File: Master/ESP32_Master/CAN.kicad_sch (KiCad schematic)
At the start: 6 parts, among them U11 ISO1050DUBR

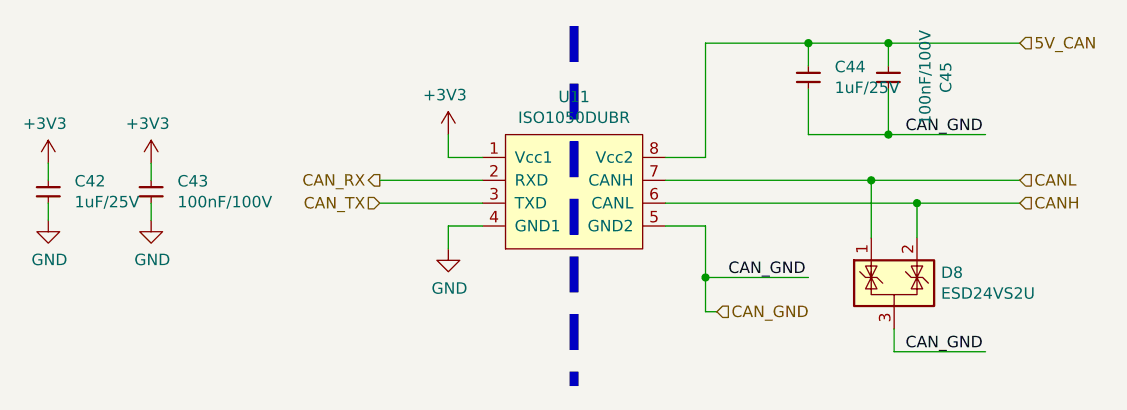
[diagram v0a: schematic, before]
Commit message: Add files via upload
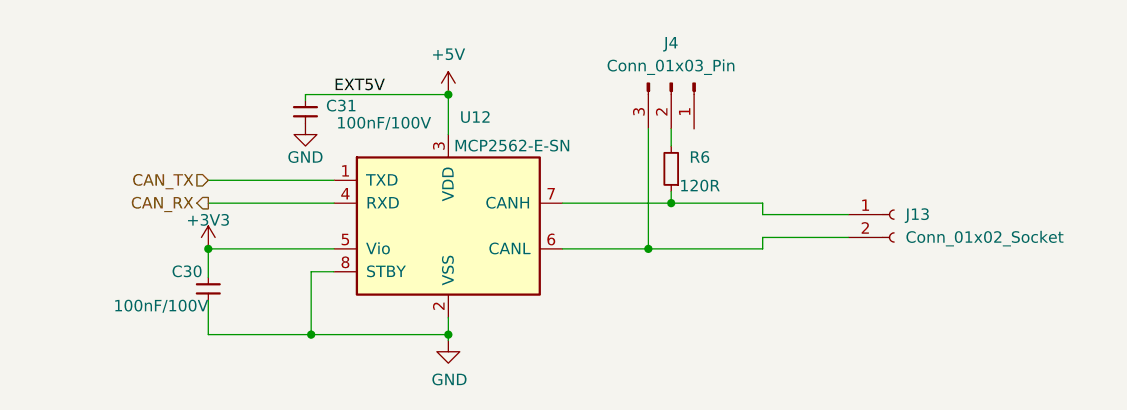
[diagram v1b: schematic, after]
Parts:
- removed C42, C44: 1uF/25V, Capacitor_SMD:C_0603_1608Metric, symbol Device:C
- removed C43, C45: 100nF/100V, Capacitor_SMD:C_0603_1608Metric, symbol Device:C
- removed D8: ESD24VS2U, Package_TO_SOT_SMD:SOT-23, symbol Power_Protection:SZNUP2105L
- removed U11: ISO1050DUBR, Package_SO:SOP-8_6.62x9.15mm_P2.54mm, symbol ENNOID:ISO1050DUBR
- added C30, C31: 100nF/100V, Capacitor_SMD:C_0603_1608Metric, symbol Device:C
- added J13: Conn_01x02_Socket, Connector_PinSocket_2.54mm:PinSocket_1x02_P2.54mm_Vertical, symbol Connector:Conn_01x02_Socket
- added J4: Conn_01x03_Pin, Connector_PinHeader_2.54mm:PinHeader_1x03_P2.54mm_Vertical, symbol Connector:Conn_01x03_Pin
- added R6: 120R, Resistor_SMD:R_0603_1608Metric, symbol Device:R_Small
- added U12: MCP2562-E-SN, Package_SO:SOIC-8_3.9x4.9mm_P1.27mm, symbol Interface_CAN_LIN:MCP2562-E-SN
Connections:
- net +3V3: now also C30.2, U12.5 (Vio)
- net CAN_RX: now also U12.4 (RXD)
- net CAN_TX: now also U12.1 (TXD)
- net GND: now also C30.1, C31.1, U12.2 (VSS), U12.8 (STBY)
- new net: J13.2 (Pin_2), J4.3 (Pin_3), U12.6 (CANL)
- new net: J13.1 (Pin_1), R6.1, U12.7 (CANH)
- new net: J4.2 (Pin_2), R6.2
- new net +5V: C31.2, U12.3 (VDD)

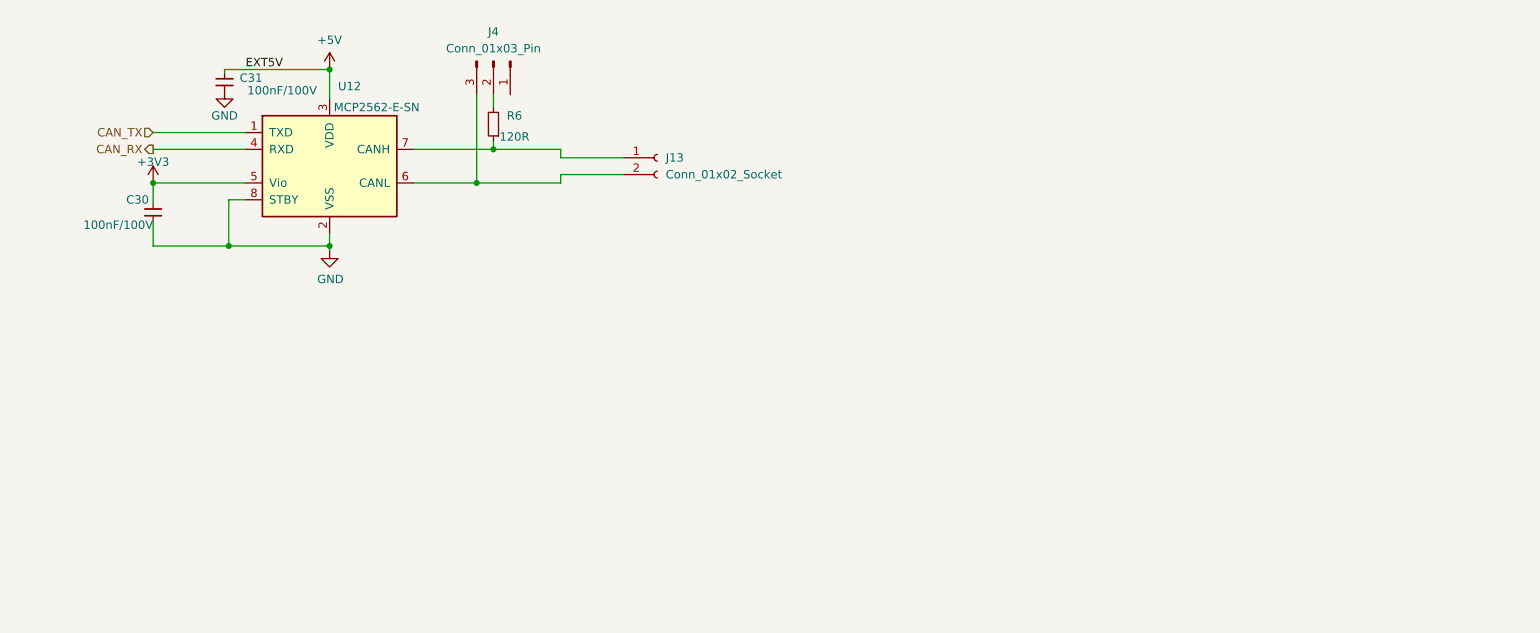
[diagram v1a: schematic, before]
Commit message: Add files via upload
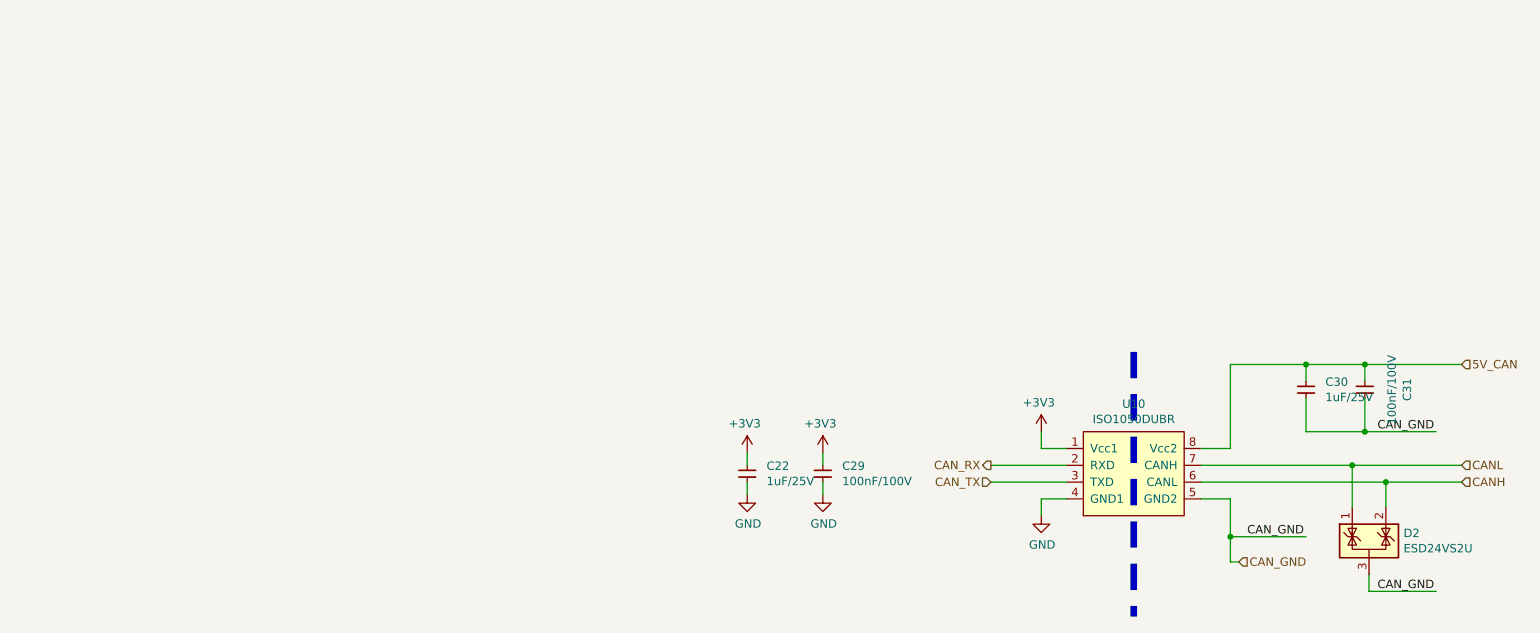
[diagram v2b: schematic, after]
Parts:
- removed J13: Conn_01x02_Socket, Connector_PinSocket_2.54mm:PinSocket_1x02_P2.54mm_Vertical, symbol Connector:Conn_01x02_Socket
- removed J4: Conn_01x03_Pin, Connector_PinHeader_2.54mm:PinHeader_1x03_P2.54mm_Vertical, symbol Connector:Conn_01x03_Pin
- removed R6: 120R, Resistor_SMD:R_0603_1608Metric, symbol Device:R_Small
- removed U12: MCP2562-E-SN, Package_SO:SOIC-8_3.9x4.9mm_P1.27mm, symbol Interface_CAN_LIN:MCP2562-E-SN
- added C22: 1uF/25V, Capacitor_SMD:C_0603_1608Metric, symbol Device:C
- added C29: 100nF/100V, Capacitor_SMD:C_0603_1608Metric, symbol Device:C
- added D2: ESD24VS2U, Package_TO_SOT_SMD:SOT-23, symbol Power_Protection:SZNUP2105L
- added U10: ISO1050DUBR, Package_SO:SOP-8_6.62x9.15mm_P2.54mm, symbol ENNOID:ISO1050DUBR
- C30: value 100nF/100V -> 1uF/25V; Link https://www.digikey.jp/en/products/detail/samsung-electro-m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 -> https://www.digikey.jp/en/products/detail/nextgen-component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; MPN CL10B104KC8NNNC -> 0603B105K250XD
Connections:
- net +3V3: now also C22.1, C29.1, U10.1 (Vcc1); no longer C30.2
- net CAN_RX: now also U10.2 (RXD)
- net CAN_TX: now also U10.3 (TXD)
- net GND: now also C22.2, C29.2, U10.4 (GND1); no longer C30.1, C31.1
- net +5V renamed 5V_CAN
- net 5V_CAN: now also C30.1, U10.8 (Vcc2)
- new net CANH: D2.2 (K), U10.6 (CANL)
- new net CANL: D2.1 (K), U10.7 (CANH)
- new net CAN_GND: C30.2, C31.1, D2.3 (A), U10.5 (GND2)
